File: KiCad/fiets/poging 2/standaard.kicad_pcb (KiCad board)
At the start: 2 copper layers, 95.2 x 57.1 mm, 24 parts, among them J1 Conn_01x04_Female, J2 R pinnen RGB strips, J3 282837-4, J4 282841-2, J5 282841-2, SW1 ENABLE, SW2 BOOT, U1 ESP32-WROOM-32E_(16MB)

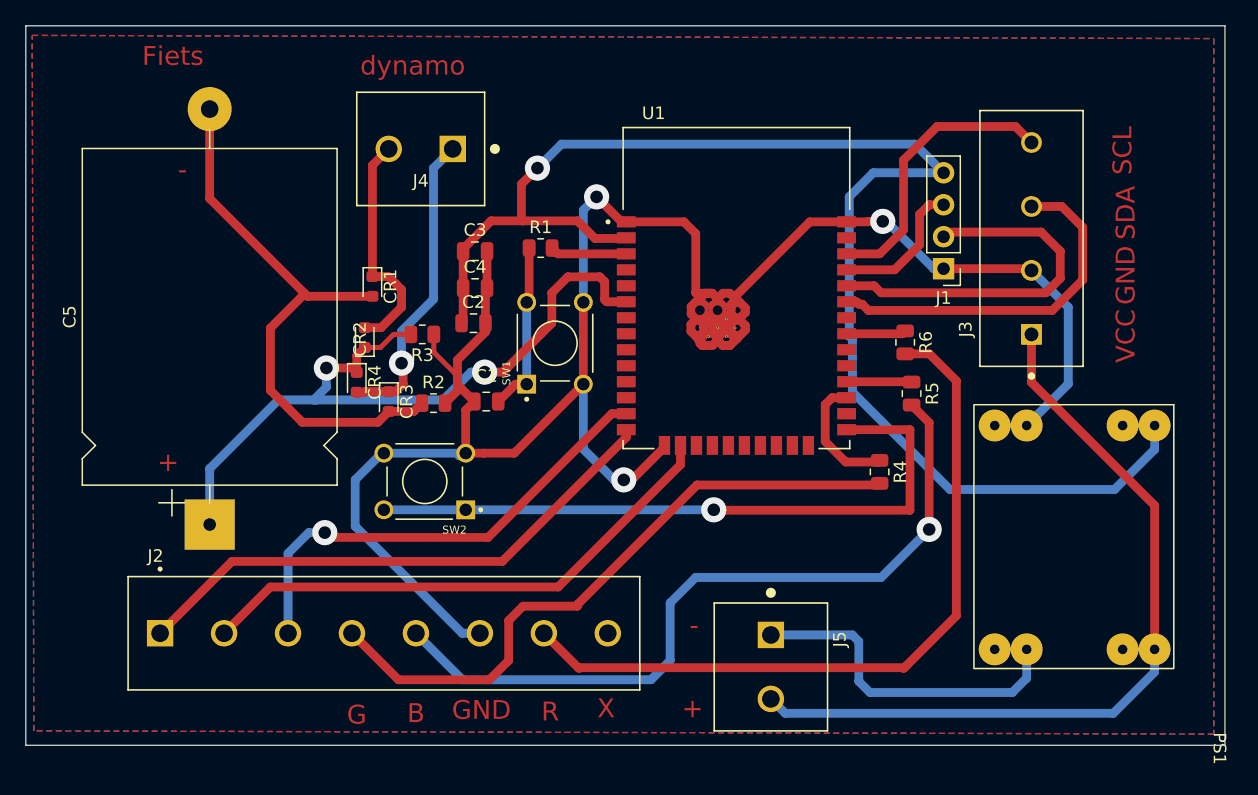
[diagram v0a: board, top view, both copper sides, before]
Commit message: betere versie kicad fiets
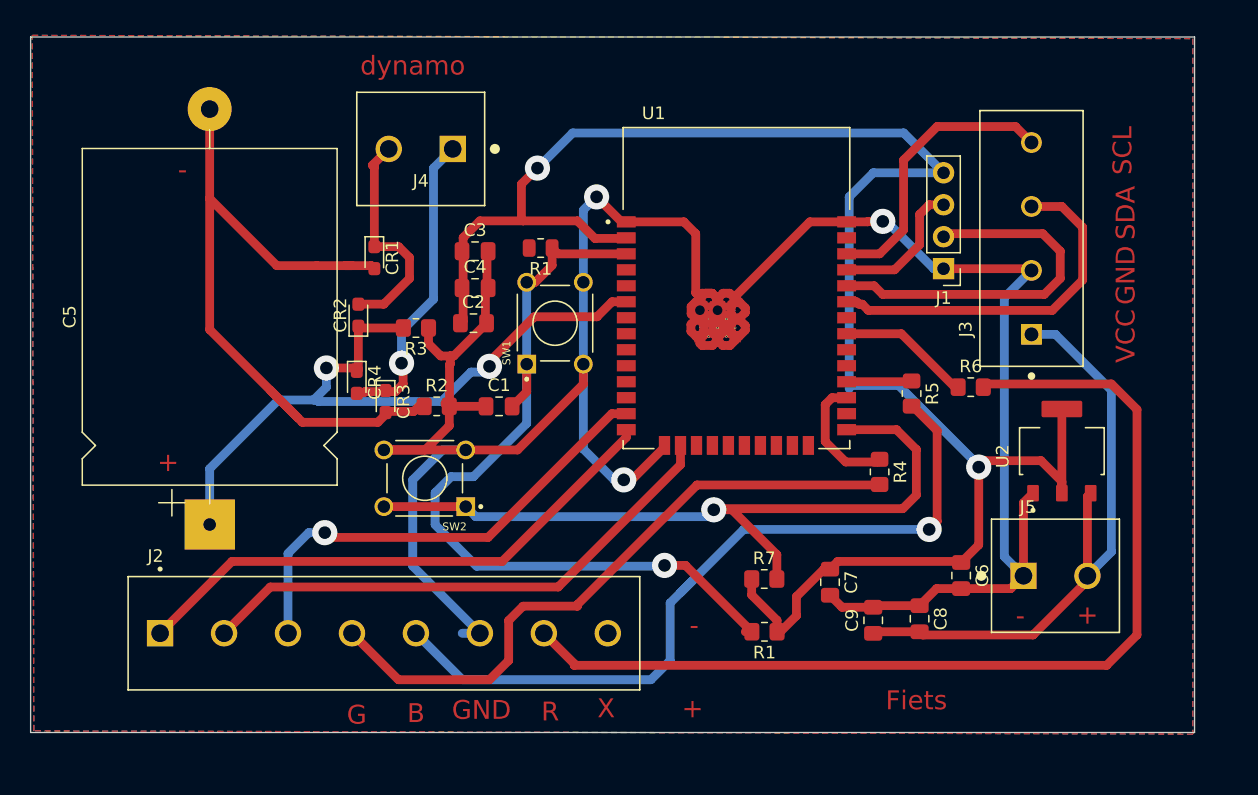
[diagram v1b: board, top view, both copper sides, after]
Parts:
- removed PS1: ITX0512SA, libraries:Buck Converter
- added C6: 0.1u, Capacitor_SMD:C_0805_2012Metric_Pad1.18x1.45mm_HandSolder, F.Cu at (194.3, 70.2)
- added C7: 4.7u, Capacitor_SMD:C_0805_2012Metric_Pad1.18x1.45mm_HandSolder, F.Cu at (183.9, 70.7)
- added C8: 0.1u, Capacitor_SMD:C_0805_2012Metric_Pad1.18x1.45mm_HandSolder, F.Cu at (191.0, 73.6)
- added C9: 4.7u, Capacitor_SMD:C_0805_2012Metric_Pad1.18x1.45mm_HandSolder, F.Cu at (187.3, 73.8)
- added R1: 10k, Resistor_SMD:R_0805_2012Metric_Pad1.20x1.40mm_HandSolder, F.Cu at (178.7, 74.7)
- added R7: 10k, Resistor_SMD:R_0805_2012Metric_Pad1.20x1.40mm_HandSolder, F.Cu at (178.7, 70.5)
- added U2: AMS1117, libraries:SOT229P700X180-4N, F.Cu at (202.3, 60.3)
- C1, C2, C3, C4: footprint Capacitor_SMD:C_0805_2012Metric -> Capacitor_SMD:C_0805_2012Metric_Pad1.18x1.45mm_HandSolder
- CR1, CR2, CR3, CR4: footprint Diode_SMD:D_0603_1608Metric -> Diode_SMD:D_0603_1608Metric_Pad1.05x0.95mm_HandSolder
- R2, R3, R4, R5, R6: footprint Resistor_SMD:R_0805_2012Metric -> Resistor_SMD:R_0805_2012Metric_Pad1.20x1.40mm_HandSolder
- moved J5 23.7 mm to (201.8, 70.2), turned to 0 degrees
- moved R6 6.31 mm to (195.1, 55.2), turned to 0 degrees
- moved CR1 2.29 mm to (147.7, 45.0)
- moved CR2 1.85 mm to (146.4, 49.5)
- moved SW1 1.59 mm to (162.1, 50.2)
- moved C1 1.09 mm to (157.6, 56.8)
- moved R3 0.72 mm to (151.0, 50.5)
- moved R2 0.36 mm to (152.7, 56.8)
- moved SW2 0.25 mm to (151.7, 62.5)
- moved CR3 0.25 mm to (148.6, 56.4)
- turned R1 to 180 degrees
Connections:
- net Net-(C2-Pad1) renamed +3V3
- net Net-(J3-Pad1) renamed 5V
- J5 pad 1: Net-(J5-Pad1) -> GND
- U1 pad 3: Net-(R1-Pad2) -> Net-(C1-Pad2)
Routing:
- net Net-(C1-Pad2): track 13.7 -> 67.5 mm, vias 0 -> 1
- net GND: track 187.8 -> 226.2 mm
- net +3V3: track 114.7 -> 144.1 mm, vias 1 -> 2
- net Net-(J5-Pad1): track 26.8 -> 0.00 mm
- net Net-(J2-Pad7): track 59.6 -> 80.3 mm
- net 5V: track 63.2 -> 49.7 mm
- net Net-(C5-Pad2): track 45.8 -> 57.0 mm
- net Net-(R7-Pad2): track 53.4 -> 61.7 mm
- net Net-(R1-Pad2): track 6.08 -> 0.00 mm
- net Net-(R6-Pad1): track 4.75 -> 10.6 mm
- net Net-(C5-Pad1): track 59.2 -> 55.9 mm
- net Net-(J2-Pad5): track 60.6 -> 62.9 mm
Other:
- board size 95.2 x 57.1 mm -> 92.5 x 55.2 mm
